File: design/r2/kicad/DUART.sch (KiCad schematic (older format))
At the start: 12 parts, among them IC4 XR68C681CJTR-F, J1 UART_A, J2 UART_B, J4 Conn_01x06, Q1 Crystal

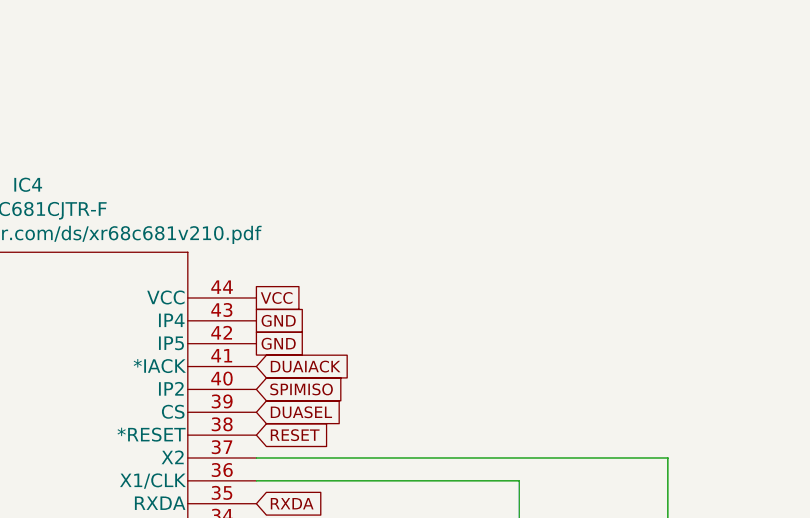
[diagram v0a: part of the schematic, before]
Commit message: Tidy up footprints
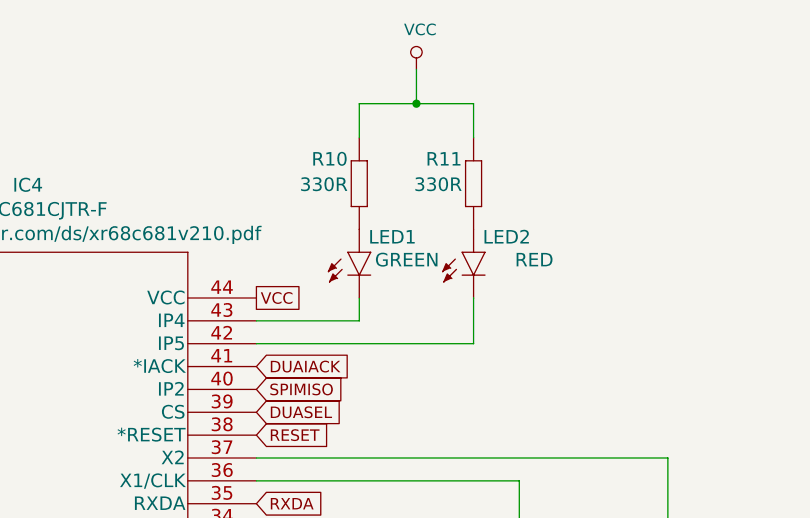
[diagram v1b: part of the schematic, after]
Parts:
- added LED1: GREEN, rosco_m68k:LED5MM, symbol rosco_m68k-eagle-import:LED5MM
- added LED2: RED, rosco_m68k:LED5MM, symbol rosco_m68k-eagle-import:LED5MM
- added R10, R11: 330R, rosco_m68k:0207_10, symbol rosco_m68k-eagle-import:R-EU_0207_10
- C1, C2: footprint Capacitor_THT:C_Rect_L7.0mm_W2.0mm_P5.00mm -> rosco_m68k:C2.5-3
- J1, J2: footprint Connector_PinHeader_2.54mm:PinHeader_1x06_P2.54mm_Vertical -> rosco_m68k:1X06
- JP1, JP2: footprint Connector_PinHeader_2.54mm:PinHeader_1x02_P2.54mm_Vertical -> rosco_m68k:1X02
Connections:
- wire segments 32 -> 41
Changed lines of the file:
@@
 $Descr A4 11693 8268
 encoding utf-8
-Sheet 4 7
+Sheet 3 7
 Title "ROSCO_M68K GENERAL PURPOSE MC68010 COMPUTER"
 Date "2021-10-08"
@@
 F 0 "C1" H 7665 3896 50  0000 L CNN
 F 1 "7pF" H 7665 3805 50  0000 L CNN
-F 2 "Capacitor_THT:C_Rect_L7.0mm_W2.0mm_P5.00mm" H 7588 3700 50  0001 C CNN
+F 2 "rosco_m68k:C2.5-3" H 7588 3700 50  0001 C CNN
 F 3 "~" H 7550 3850 50  0001 C CNN
 	1    7550 3850
@@
 F 0 "C2" H 8315 3896 50  0000 L CNN
 F 1 "7pF" H 8315 3805 50  0000 L CNN
-F 2 "Capacitor_THT:C_Rect_L7.0mm_W2.0mm_P5.00mm" H 8238 3700 50  0001 C CNN
+F 2 "rosco_m68k:C2.5-3" H 8238 3700 50  0001 C CNN
 F 3 "~" H 8200 3850 50  0001 C CNN
 	1    8200 3850
@@
 F 0 "J1" H 1358 6231 50  0000 C CNN
 F 1 "UART_A" H 1358 6140 50  0000 C CNN
-F 2 "Connector_PinHeader_2.54mm:PinHeader_1x06_P2.54mm_Vertical" H 1250 5850 50  0001 C CNN
+F 2 "rosco_m68k:1X06" H 1250 5850 50  0001 C CNN
 F 3 "~" H 1250 5850 50  0001 C CNN
 	1    1250 5850
@@
 F 0 "J2" H 1358 7081 50  0000 C CNN
 F 1 "UART_B" H 1358 6990 50  0000 C CNN
-F 2 "Connector_PinHeader_2.54mm:PinHeader_1x06_P2.54mm_Vertical" H 1250 6700 50  0001 C CNN
+F 2 "rosco_m68k:1X06" H 1250 6700 50  0001 C CNN
 F 3 "~" H 1250 6700 50  0001 C CNN
 	1    1250 6700
@@
 NoConn ~ 4400 3300
 NoConn ~ 4400 3400
-Text GLabel 6400 1900 2    50   UnSpc ~ 0
-GND
-Text GLabel 6400 2000 2    50   UnSpc ~ 0
-GND
 Text GLabel 4400 2000 0    50   UnSpc ~ 0
 GND
@@
 F 0 "JP2" H 10000 5914 50  0000 C CNN
 F 1 "Jumper" H 10000 5823 50  0000 C CNN
-F 2 "Connector_PinHeader_2.54mm:PinHeader_1x02_P2.54mm_Vertical" H 10000 5650 50  0001 C CNN
+F 2 "rosco_m68k:1X02" H 10000 5650 50  0001 C CNN
 F 3 "~" H 10000 5650 50  0001 C CNN
 	1    10000 5650
@@
 F 0 "JP1" H 10000 5464 50  0000 C CNN
 F 1 "Jumper" H 10000 5373 50  0000 C CNN
-F 2 "Connector_PinHeader_2.54mm:PinHeader_1x02_P2.54mm_Vertical" H 10000 5200 50  0001 C CNN
+F 2 "rosco_m68k:1X02" H 10000 5200 50  0001 C CNN
 F 3 "~" H 10000 5200 50  0001 C CNN
 	1    10000 5200
@@
 Text GLabel 1450 7000 2    50   Input ~ 0
 RTSB
+$Comp
+L rosco_m68k-eagle-import:R-EU_0207_10 R?
+U 1 1 6161B40D
+P 6850 1300
+AR Path="/6161B40D" Ref="R?"  Part="1"
+AR Path="/5E53B952/6161B40D" Ref="R?"  Part="1"
+AR Path="/60FBFA5C/6161B40D" Ref="R?"  Part="1"
+AR Path="/61043B8D/6161B40D" Ref="R?"  Part="1"
+AR Path="/6162E38E/6161B40D" Ref="R?"  Part="1"
+AR Path="/61622E90/6161B40D" Ref="R10"  Part="1"
+F 0 "R10" V 6991 1350 59  0000 L BNN
+F 1 "330R" V 6880 1350 59  0000 L BNN
+F 2 "rosco_m68k:0207_10" H 6850 1300 50  0001 C CNN
+F 3 "" H 6850 1300 50  0001 C CNN
+	1    6850 1300
+	0    -1   -1   0
+$EndComp
+$Comp
+L rosco_m68k-eagle-import:LED5MM LED?
+U 1 1 6161B413
+P 6850 1600
+AR Path="/6161B413" Ref="LED?"  Part="1"
+AR Path="/5E53B952/6161B413" Ref="LED?"  Part="1"
+AR Path="/60FBFA5C/6161B413" Ref="LED?"  Part="1"
+AR Path="/61043B8D/6161B413" Ref="LED?"  Part="1"
+AR Path="/6162E38E/6161B413" Ref="LED?"  Part="1"
+AR Path="/61622E90/6161B413" Ref="LED1"  Part="1"
+F 0 "LED1" H 7100 1700 59  0000 R TNN
+F 1 "GREEN" H 7200 1600 59  0000 R TNN
+F 2 "rosco_m68k:LED5MM" H 6850 1600 50  0001 C CNN
+F 3 "" H 6850 1600 50  0001 C CNN
+	1    6850 1600
+	1    0    0    -1
+$EndComp
+$Comp
+L rosco_m68k-eagle-import:R-EU_0207_10 R?
+U 1 1 6161C7AA
+P 7350 1300
+AR Path="/6161C7AA" Ref="R?"  Part="1"
+AR Path="/5E53B952/6161C7AA" Ref="R?"  Part="1"
+AR Path="/60FBFA5C/6161C7AA" Ref="R?"  Part="1"
+AR Path="/61043B8D/6161C7AA" Ref="R?"  Part="1"
+AR Path="/6162E38E/6161C7AA" Ref="R?"  Part="1"
+AR Path="/61622E90/6161C7AA" Ref="R11"  Part="1"
+F 0 "R11" V 7491 1350 59  0000 L BNN
+F 1 "330R" V 7380 1350 59  0000 L BNN
+F 2 "rosco_m68k:0207_10" H 7350 1300 50  0001 C CNN
+F 3 "" H 7350 1300 50  0001 C CNN
+	1    7350 1300
+	0    -1   -1   0
+$EndComp
+$Comp
+L rosco_m68k-eagle-import:LED5MM LED?
+U 1 1 6161C7B0
+P 7350 1600
+AR Path="/6161C7B0" Ref="LED?"  Part="1"
+AR Path="/5E53B952/6161C7B0" Ref="LED?"  Part="1"
+AR Path="/60FBFA5C/6161C7B0" Ref="LED?"  Part="1"
+AR Path="/61043B8D/6161C7B0" Ref="LED?"  Part="1"
+AR Path="/6162E38E/6161C7B0" Ref="LED?"  Part="1"
+AR Path="/61622E90/6161C7B0" Ref="LED2"  Part="1"
+F 0 "LED2" H 7600 1700 59  0000 R TNN
+F 1 "RED" H 7700 1600 59  0000 R TNN
+F 2 "rosco_m68k:LED5MM" H 7350 1600 50  0001 C CNN
+F 3 "" H 7350 1600 50  0001 C CNN
+	1    7350 1600
+	1    0    0    -1
+$EndComp
+Wire Wire Line
+	6400 1900 6850 1900
+Wire Wire Line
+	6850 1900 6850 1800
+Wire Wire Line
+	6400 2000 7350 2000
+Wire Wire Line
+	7350 2000 7350 1800
+$Comp
+L power:VCC #PWR04
+U 1 1 6161F2BF
+P 7100 800
+F 0 "#PWR04" H 7100 650 50  0001 C CNN
+F 1 "VCC" H 7117 973 50  0000 C CNN
+F 2 "" H 7100 800 50  0001 C CNN
+F 3 "" H 7100 800 50  0001 C CNN
+	1    7100 800
+	1    0    0    -1
+$EndComp
+Wire Wire Line
+	6850 1100 6850 950
+Wire Wire Line
+	6850 950  7100 950
+Wire Wire Line
+	7100 950  7100 800
+Wire Wire Line
+	7350 1100 7350 950
+Wire Wire Line
+	7350 950  7100 950
+Connection ~ 7100 950
 $EndSCHEMATC
